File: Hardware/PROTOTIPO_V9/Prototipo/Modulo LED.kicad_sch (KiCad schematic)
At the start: 5 parts, among them J4 Conn_01x06, J7 Conn_01x01, J8 Conn_01x06, J9 Conn_01x01, U9 CR2013-MI2120

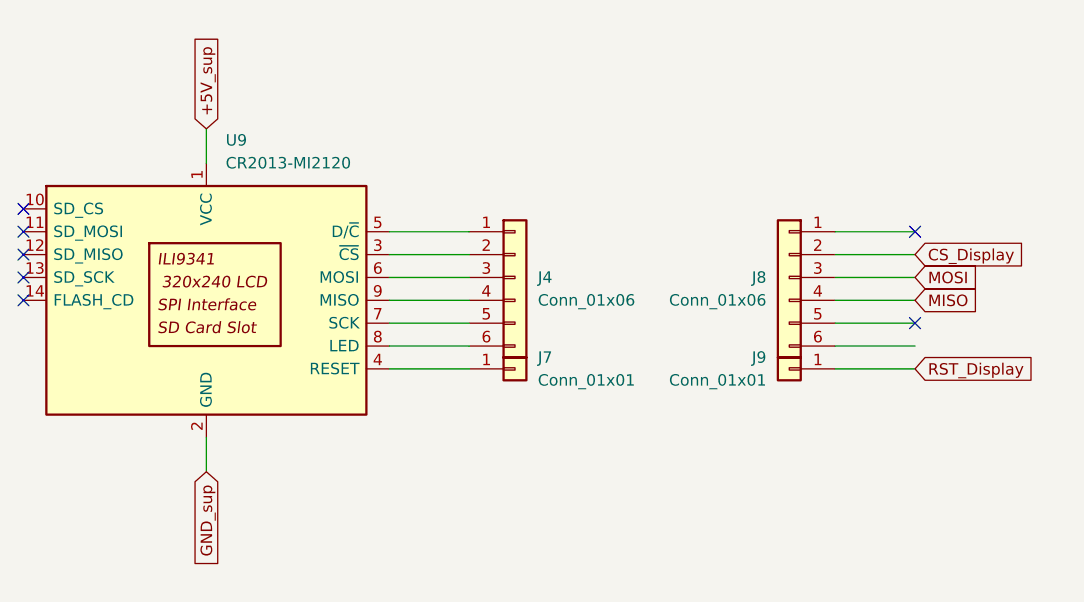
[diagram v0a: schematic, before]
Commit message: Bus de salida
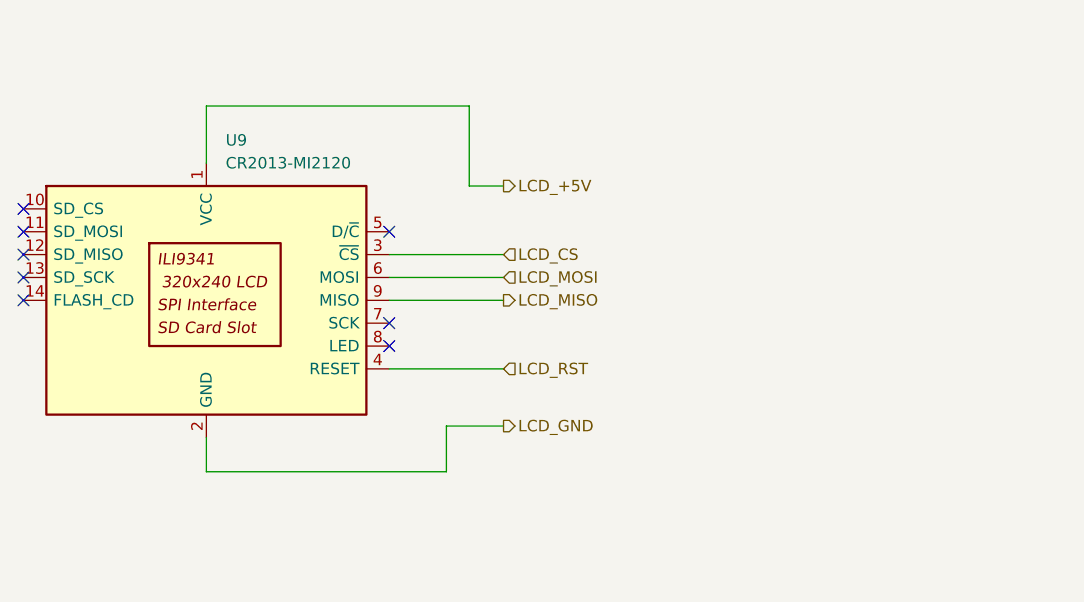
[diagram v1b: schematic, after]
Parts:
- removed J4, J8: Conn_01x06, symbol Connector_Generic:Conn_01x06
- removed J7, J9: Conn_01x01, symbol Connector_Generic:Conn_01x01
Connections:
- net LCD_CS: now reaches U9.3 (~{CS})
- net LCD_RST: now reaches U9.4 (RESET)
- net LCD_MOSI: now reaches U9.6 (MOSI)
- net LCD_MISO: now reaches U9.9 (MISO)
- net +5V_sup renamed LCD_+5V
- net GND_sup renamed LCD_GND
- no-connect marks 7 -> 8
